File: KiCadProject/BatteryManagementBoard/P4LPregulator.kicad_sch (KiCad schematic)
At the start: 6 parts, among them U401 BD433M5FP

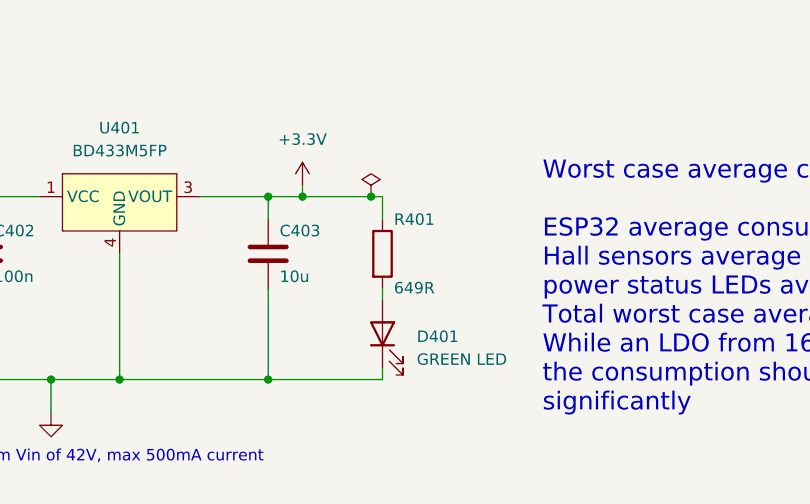
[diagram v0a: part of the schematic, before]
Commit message: Layout on the battery management board
Signed-off-by: Eldalote.Electronics <Eldalote.Electronics@gmail.com>
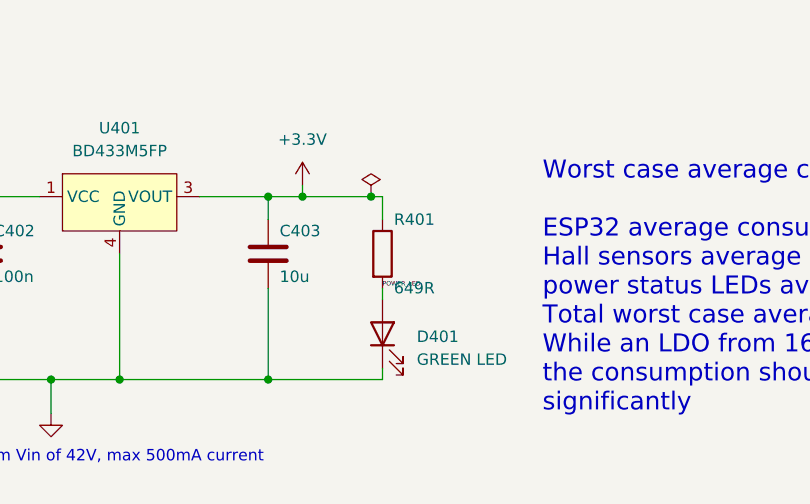
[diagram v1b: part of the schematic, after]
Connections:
- net POWER_LED: now reaches D401.2 (A), R401.2
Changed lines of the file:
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@@
     (effects (font (size 4 4) (thickness 0.8) bold) (justify left bottom))
+  )
+  (label "POWER_LED" (at 163.83 101.6 0)
+    (effects (font (size 0.5 0.5)) (justify left bottom))
   )
   (global_label "VOUT" (shape input) (at 92.71 91.44 180) (fields_autoplaced)
